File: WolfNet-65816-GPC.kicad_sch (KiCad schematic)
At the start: 38 parts, among them J1 Conn_01x01, J2 Conn_01x01, J3 Conn_01x01, J4 Conn_01x01, J5 USB_B, J6 ATX-24, SW1 SW_SPST, SW2 SW_Push, U1 WD65C816S, U10 LM7905_TO220, U11 SC28L91, U12 DS1813, U2 MCP2200-I-SO, U3 74HCT573, U4 74HCT245, U5 AS6C1608, U6 XCR3064XL-VQ100, U7 SST39SF040, U8 SST39SF040, U9 XCR3064XL-VQ100, X1 ACO-12MHz, X2 ACO-3.6864MHz

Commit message: Update WolfNet-65816-GPC.kicad_sch
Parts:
- removed U6: XCR3064XL-VQ100, Package_QFP:LQFP-100_14x14mm_P0.5mm, symbol CPLD_Xilinx:XCR3064XL-VQ100
- added J?: 65SIB_Connector, symbol Connector (Open HW):65SIB_Connector
- added U?: XCR3256XL-TQ144, Package_QFP:TQFP-144_20x20mm_P0.5mm, symbol CPLD_Xilinx:XCR3256XL-TQ144
- added U?: 74HCT137, symbol 74xx:74HCT137
- added U?: 28C16, symbol Memory:28C16
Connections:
- net +12V: now also J?.10 (12v), J?.8 (12v)
- net +5V: now also U?.20 (VCC), U?.115 (VCC), U?.123 (VCC), U?.130 (VCC), U?.144 (VCC), U?.16 (VCC), U?.24 (VCC), U?.24 (VCC), U?.50 (VCC), U?.51 (VCC), U?.58 (VCC), U?.73 (VCC), U?.76 (VCC), U?.95 (VCC)
- net -12V: now also J?.13 (-12v)
- net A0: now also U?.38 (RS0), U?.8 (A0)
- net A1: now also U?.37 (RS1), U?.7 (A1)
- net A10: now also U?.19 (A10)
- net A2: now also U?.36 (RS2), U?.6 (A2)
- net A3: now also U?.35 (RS3), U?.5 (A3)
- net A4: now also U?.4 (A4)
- net A5: now also U?.3 (A5)
- net A6: now also U?.2 (A6)
- net A7: now also U?.1 (A7)
- net A8: now also U?.23 (A8)
- net A9: now also U?.22 (A9)
- net D0: now also U?.33 (D0), U?.9 (D0)
- net D1: now also U?.32 (D1), U?.10 (D1)
- net D2: now also U?.31 (D2), U?.11 (D2)
- net D3: now also U?.30 (D3), U?.13 (D3)
- net D4: now also U?.29 (D4), U?.14 (D4)
- net D5: now also U?.28 (D5), U?.15 (D5)
- net D6: now also U?.27 (D6), U?.16 (D6)
- net D7: now also U?.26 (D7), U?.17 (D7)
- net DMA_JTAG: now also U?.13 (PORT_EN)
- net GND: now also U?.1 (GND), J?.16 (GND), J?.19 (GND), J?.2 (GND), J?.4 (GND), J?.6 (eGND), U?.105 (GND), U?.12 (GND), U?.124 (GND), U?.129 (GND), U?.135 (GND), U?.17 (GND), U?.3 (GND), U?.33 (GND), U?.52 (GND), U?.57 (GND), U?.59 (GND), U?.64 (GND), U?.8 (GND), U?.85 (GND)
- net PHI2: now also U?.25 (PHI2), U?.128 (CLK0/IN0)
- net RESET: now also J2.1 (Pin_1), U9.62 (C0/TCK)
- net R/~{W}: now also U?.22 (R/~{W})
- net ~{IRQ}: no longer JP1.1 (A)
- net ~{READ}: now also U?.20 (~{OE})
- net ~{RESET}: now also U?.34 (~{RESET})
- net ~{WRITE}: now also U?.21 (~{WE})
- net ~{E_ROM_CS}: now reaches U9.21 (D5)
- net ~{E_ROM_CS}: now also U?.18 (~{CS})
- net ~{C22_CS2}: now reaches U9.23 (D6)
- net ~{C22_CS2}: now also U?.23 (~{CS2}), U?.5 (~{E1})
- net C22_CS1: now reaches U9.25 (D7)
- net C22_CS1: now also U?.24 (CS1), U?.6 (E2)
- net ~{65SIB_IRQ}: now reaches U9.88 (CLK2/IN2)
- net ~{65SIB_IRQ}: now also U?.21 (~{IRQ})
- net ~{UART_IRQ}: now reaches U9.89 (CLK1/IN1)
- net ~{UART_IRQ}: now also JP1.1 (A)
- net PA0: now reaches U?.2 (PA0)
- net PA1: now reaches U?.3 (PA1)
- net PA2: now reaches U?.4 (PA2)
- net ~{C22_IRQ1}: now reaches U?.40 (CA1)
- net ~{C22_IRQ1}: now also J?.9 (IRO\)
- net PA3: now reaches U?.5 (PA3)
- net ~{CONF}: now reaches U?.6 (PA4)
- net ~{CONF}: now also J?.1 (CONF\)
- net 65SIB_MOSI: now reaches U?.7 (PA5)
- net 65SIB_MOSI: now also J?.5 (MOSI)
- net 65SIB_MISO: now reaches U?.8 (PA6)
- net 65SIB_MISO: now also J?.7 (MISO)
- net 65SIB_CLK: now reaches U?.9 (PA7)
- net 65SIB_CLK: now also J?.3 (CLK)
- new net PB0: U?.1 (A0)
- new net PB1: U?.2 (A1)
- new net PB2: U?.3 (A2)
- new net PB3: U?.4 (~{LE})
- new net ~{SEL1}: J?.11 (SEL1\), U?.14 (~{Y1})
- new net ~{SEL2}: J?.12 (SEL2\), U?.13 (~{Y2})
- new net ~{SEL3}: J?.14 (SEL3\), U?.12 (~{Y3})
- new net ~{SEL4}: J?.15 (SEL4\), U?.11 (~{Y4})
- new net ~{SEL5}: J?.17 (SEL5\), U?.10 (~{Y5})
- new net ~{SEL6}: J?.18 (SEL6\), U?.9 (~{Y6})
- new net ~{SEL7}: J?.20 (SEL7\), U?.7 (~{Y7})
- no-connect marks 38 -> 39
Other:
- note added: "65C02 Compatibility"
- note added: "65SIB"
- note added: "DMA Controller"
- note removed: "Connectors"
- note removed: "Direct Memory Access Circuit"
- moved on the sheet: J1, J2, J3, R2, R3, R4, U1, U?, X2

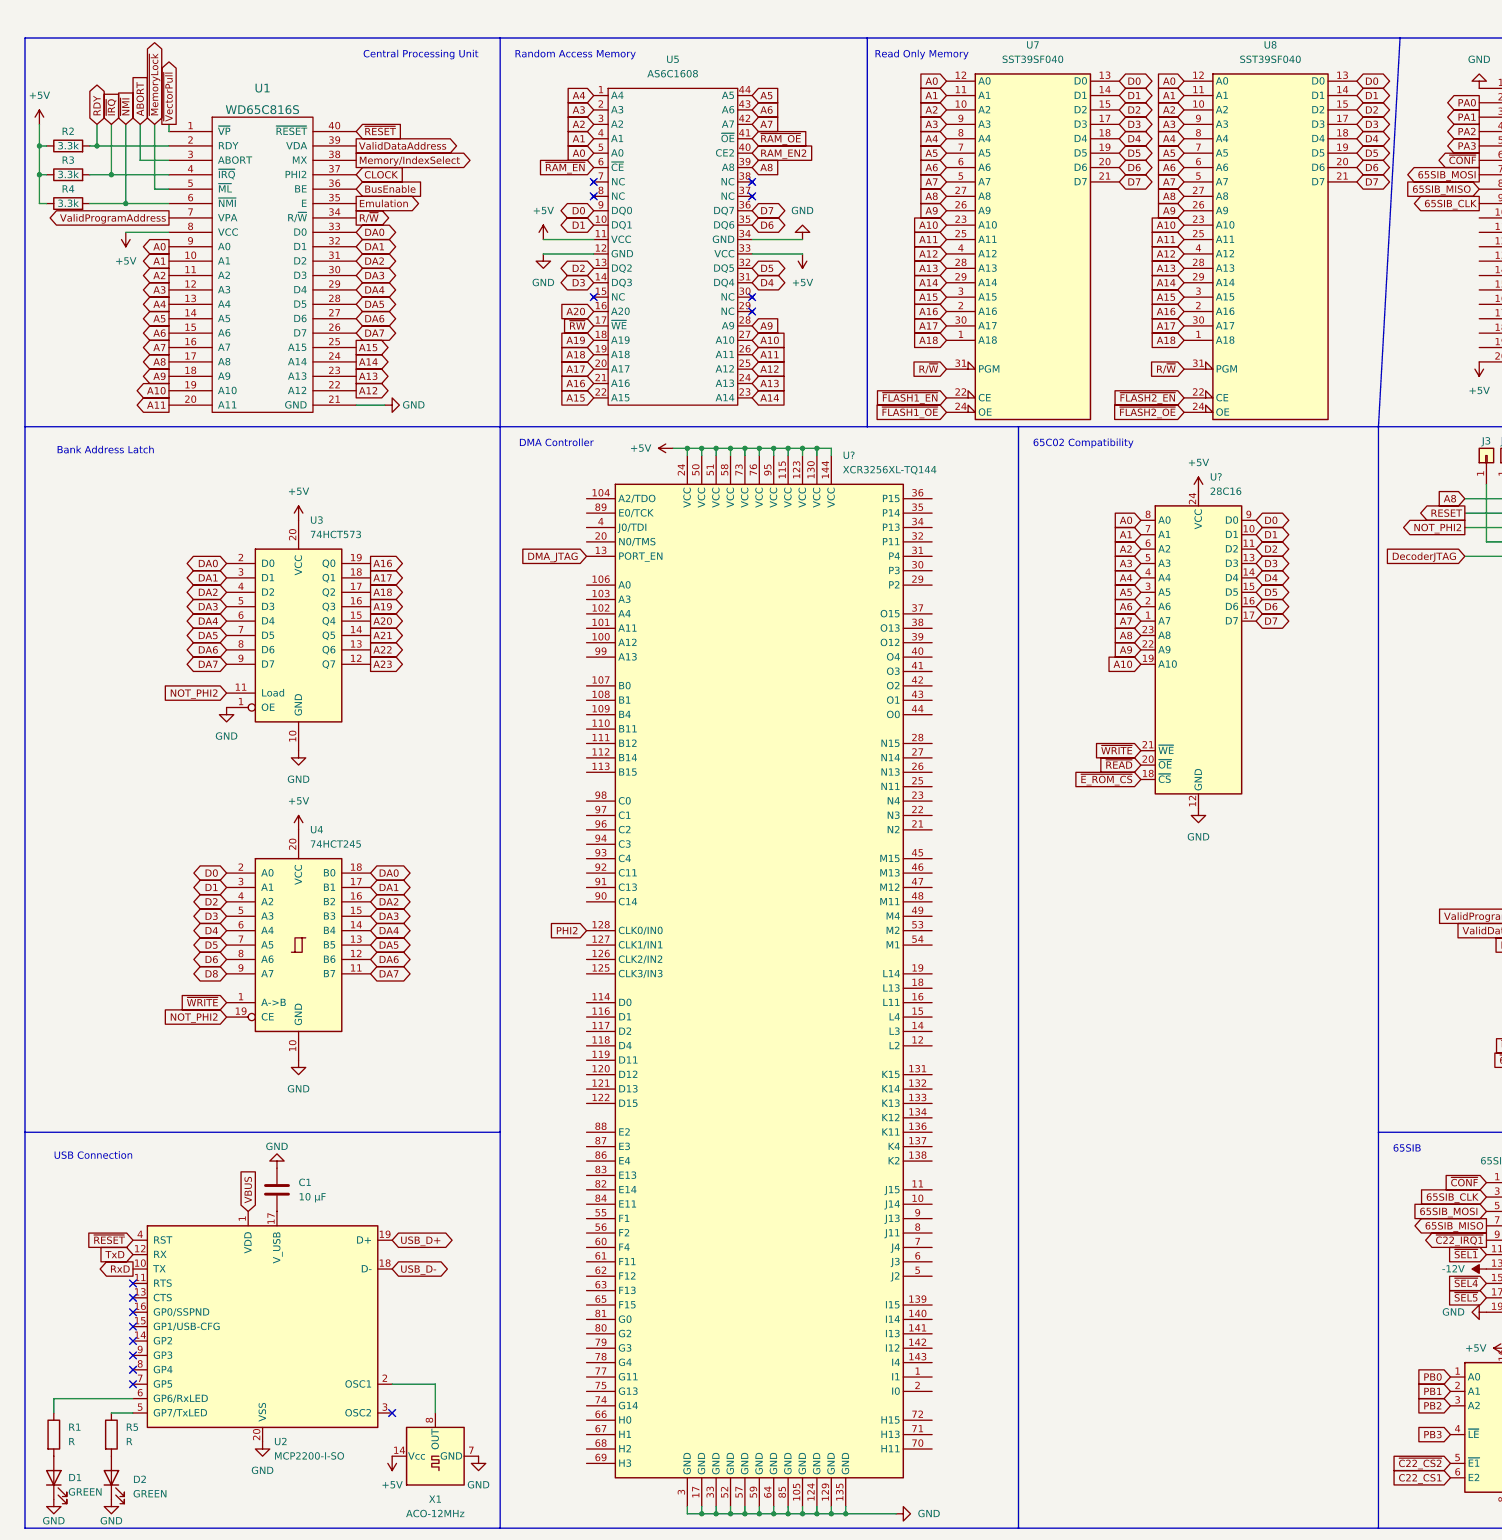
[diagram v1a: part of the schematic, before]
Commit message: Update WolfNet-65816-GPC.kicad_sch
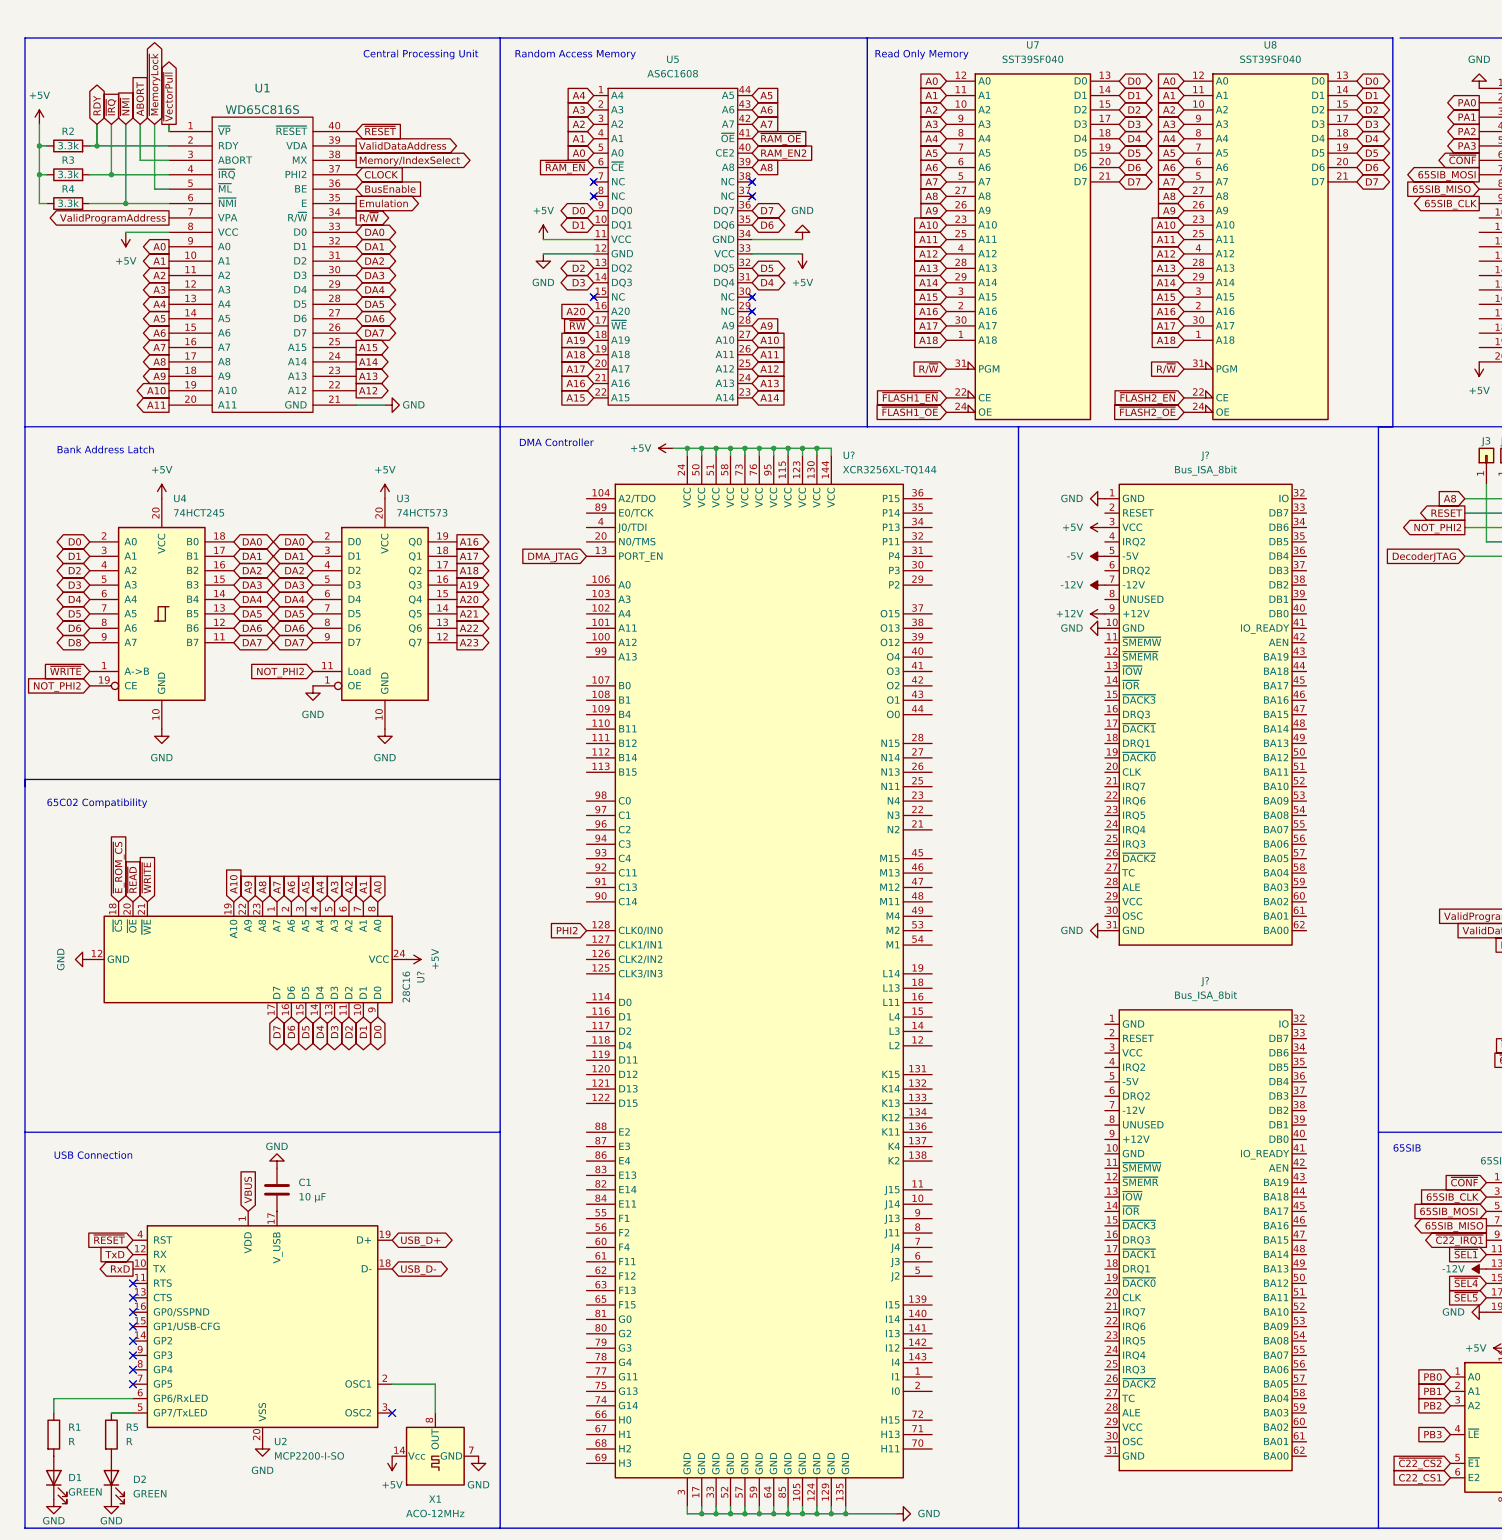
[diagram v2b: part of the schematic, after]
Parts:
- added J? (x2): Bus_ISA_8bit, symbol Connector:Bus_ISA_8bit
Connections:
- net +12V: now also J?.9 (+12V)
- net +5V: now also J?.3 (VCC)
- net -12V: now also J?.7 (-12V)
- net -5V: now also J?.5 (-5V)
- net GND: now also J?.1 (GND), J?.10 (GND), J?.31 (GND)
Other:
- moved on the sheet: U3, U4, U?
